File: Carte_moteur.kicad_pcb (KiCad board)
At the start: 2 copper layers, 112 parts, among them J101 Conn_01x02_Socket, J102 Conn_01x02, J103 Conn_01x02, J104 Conn_01x07, J105 Conn_01x02_Socket, J201 Conn_01x05_Pin, J202 Conn_01x04_Pin, J301 Conn_01x05_Pin, J302 Conn_01x04_Pin, J401 Conn_01x05_Pin, J402 Conn_01x04_Pin, J601 Conn_01x06_Pin, J602 USB_B_Mini, Q601 MMBTA44, U101 LD1117S33TR_SOT223, U201 TMC2209, U301 TMC2209, U401 TMC2209, U501 STM32G474RETx, U601 ECMF02-2AMX6, U602 LD1117S33TR_SOT223, U603 STM32F103CBTx, Y601 Crystal_GND24

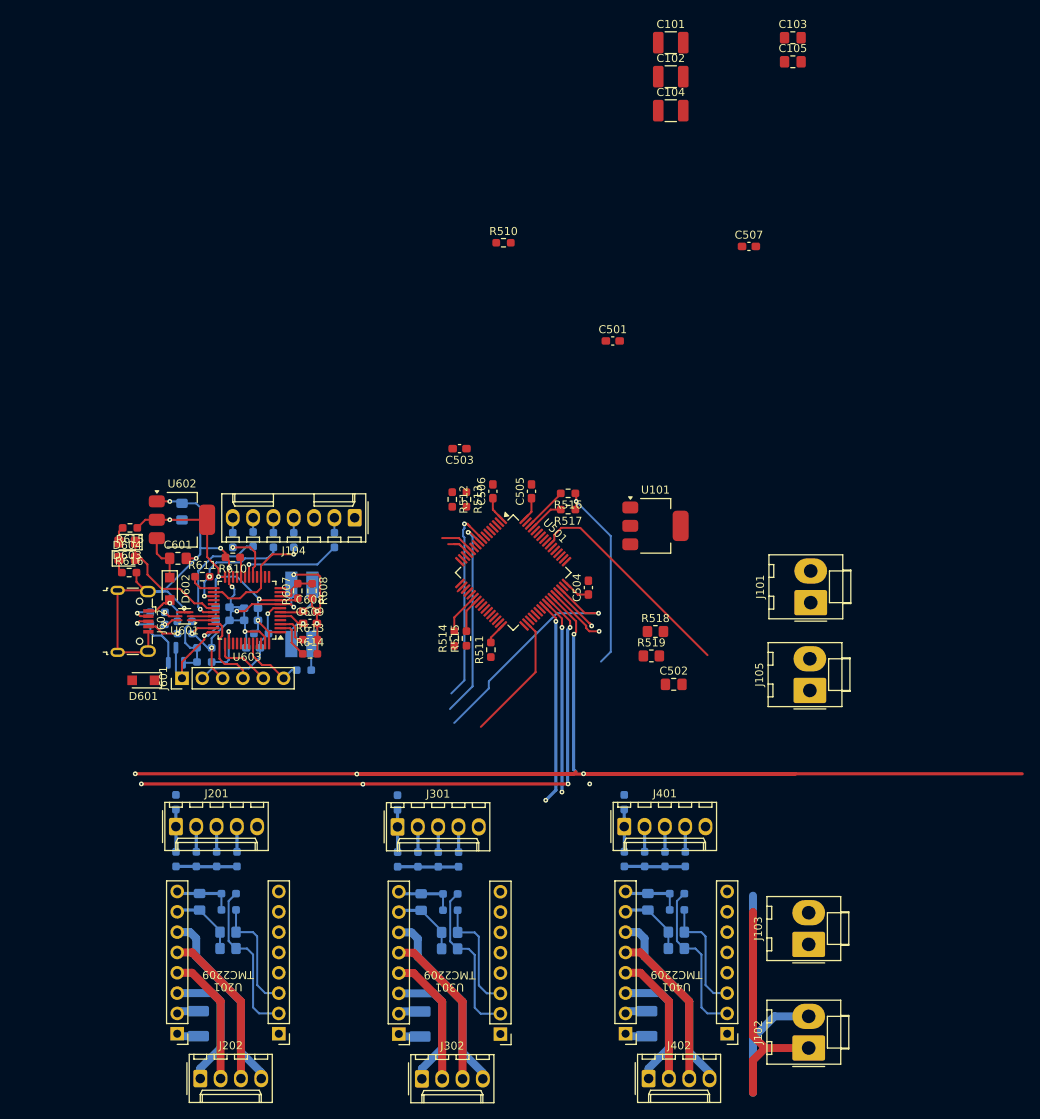
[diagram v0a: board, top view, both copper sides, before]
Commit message: before trying new µC orientation
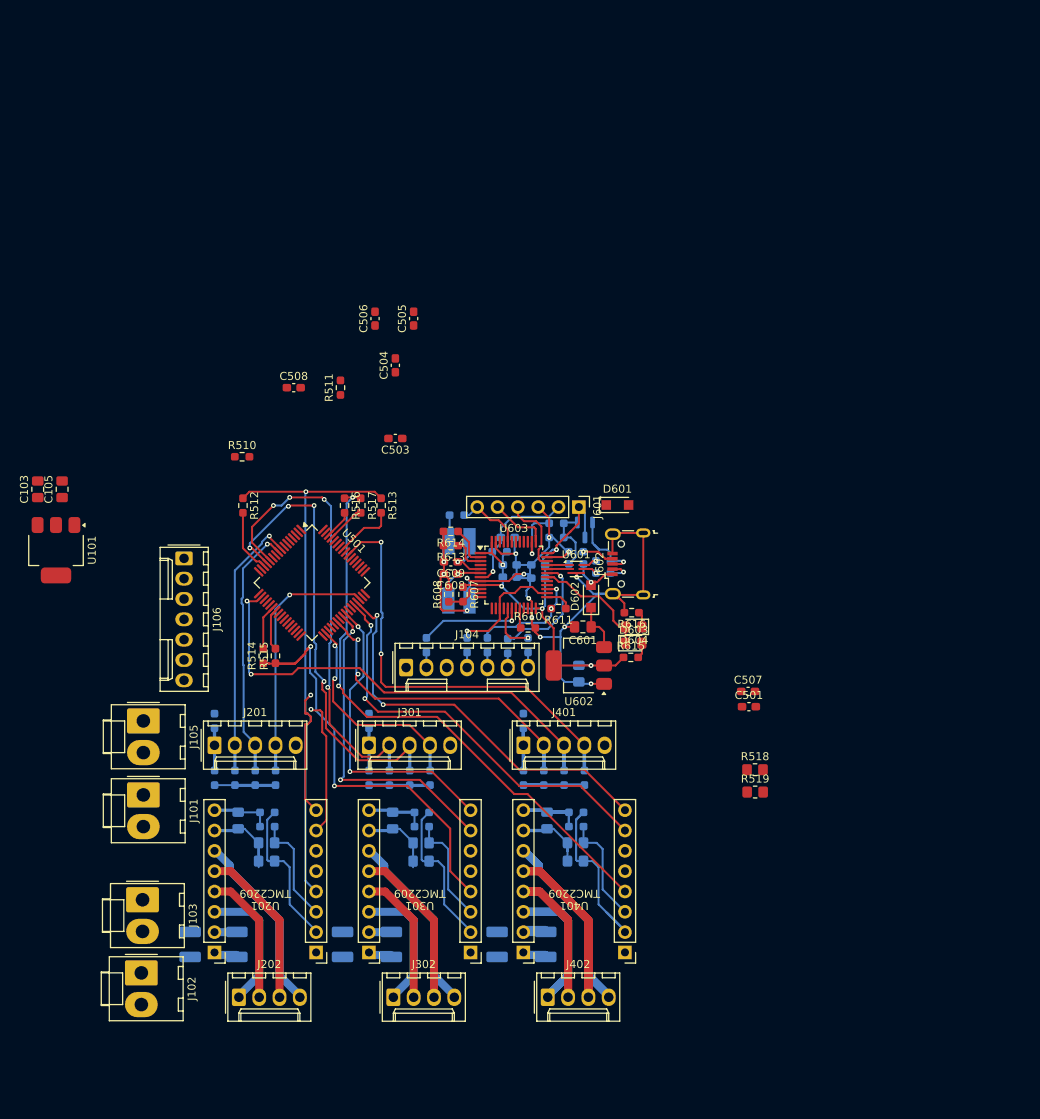
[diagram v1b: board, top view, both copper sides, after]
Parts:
- removed C502: C, Capacitor_SMD:C_0805_2012Metric_Pad1.18x1.45mm_HandSolder
- added C508: C, Capacitor_SMD:C_0603_1608Metric_Pad1.08x0.95mm_HandSolder, F.Cu at (102.1, 82.0)
- added J106: Conn_01x07, Connector_Molex:Molex_KK-254_AE-6410-07A_1x07_P2.54mm_Vertical, F.Cu at (88.4, 103.4)
- C101, C102, C104: moved to B.Cu
- moved C101 127.7 mm to (89.2, 151.6), turned to 90 degrees
- moved C102 116.0 mm to (108.2, 151.6), turned to 90 degrees
- moved C103 110.0 mm to (70.1, 94.7), turned to 90 degrees
- moved C104 106.5 mm to (127.5, 151.6), turned to 90 degrees
- moved C105 105.8 mm to (73.2, 94.7), turned to 90 degrees
- moved J101 86.8 mm to (83.3, 132.9), turned to -90 degrees
- moved J102 83.9 mm to (83.1, 155.2), turned to -90 degrees
- moved J103 83.5 mm to (83.2, 146.1), turned to -90 degrees
- moved J105 83.4 mm to (83.3, 123.7), turned to -90 degrees
- moved U101 75.0 mm to (72.4, 102.4), turned to -90 degrees
- moved R615 64.7 mm to (144.2, 115.8), turned to 0 degrees
- moved D603 64.6 mm to (144.6, 114.0), turned to 0 degrees
- moved D604 63.9 mm to (144.6, 111.9), turned to 180 degrees
- moved D601 63.2 mm to (142.6, 96.7), turned to 0 degrees
- moved R616 63.0 mm to (144.3, 110.2), turned to 180 degrees
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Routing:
- net /micro/HRTIM_CHA2: track 188.1 -> 16.1 mm, vias 4 -> 1
- net /micro/TMC1: track 0.00 -> 69.4 mm, vias 0 -> 1
- net /micro/TIM3_CH2: track 4.25 -> 64.9 mm, vias 0 -> 2
- net /micro/HRTIM_CHA1: track 77.5 -> 17.1 mm, vias 5 -> 1
- net /micro/TMC2: track 0.00 -> 56.8 mm, vias 0 -> 2
- net /micro/TIM5_CH2: track 6.98 -> 58.6 mm, vias 0 -> 4
- net /micro/TIM5_CH1: track 7.42 -> 57.4 mm, vias 0 -> 4
- net /micro/TMC3: track 24.4 -> 73.1 mm, vias 1 -> 2
- net /micro/HRTIM_CHB2: track 6.15 -> 51.1 mm, vias 1 -> 2
- net /micro/HRTIM_CHB1: track 7.78 -> 52.2 mm, vias 1 -> 2
- net /tmc_motor2/B02: track 23.6 -> 68.0 mm
- net /micro/TIM3_CH1: track 3.14 -> 45.4 mm, vias 0 -> 2
- net /tmc_motor2/B01: track 20.1 -> 60.4 mm
- net /tmc_motor2/A01: track 16.6 -> 49.7 mm
- net /tmc_motor2/A02: track 16.6 -> 49.7 mm
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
